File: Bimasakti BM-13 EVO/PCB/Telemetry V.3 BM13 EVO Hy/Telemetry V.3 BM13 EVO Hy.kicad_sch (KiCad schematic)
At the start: 7 parts, among them U1 ESP32-DEVKIT-V1, U2 74LVC125APW_118

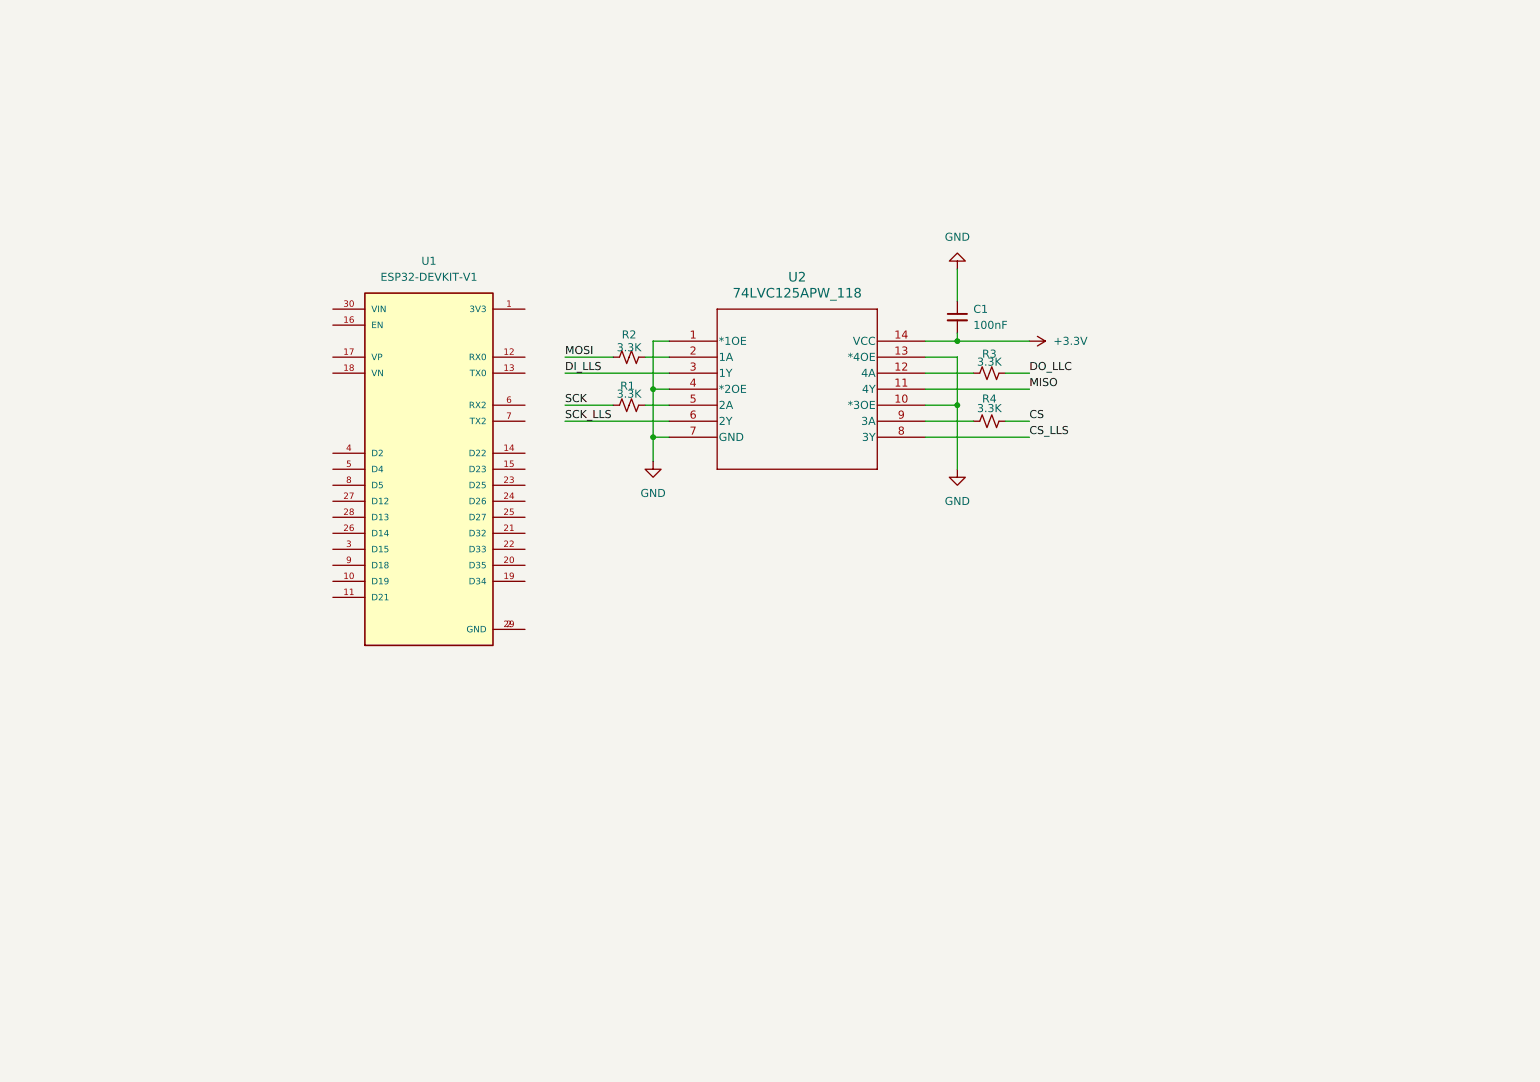
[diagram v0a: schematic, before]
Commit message: Arjun Ganti
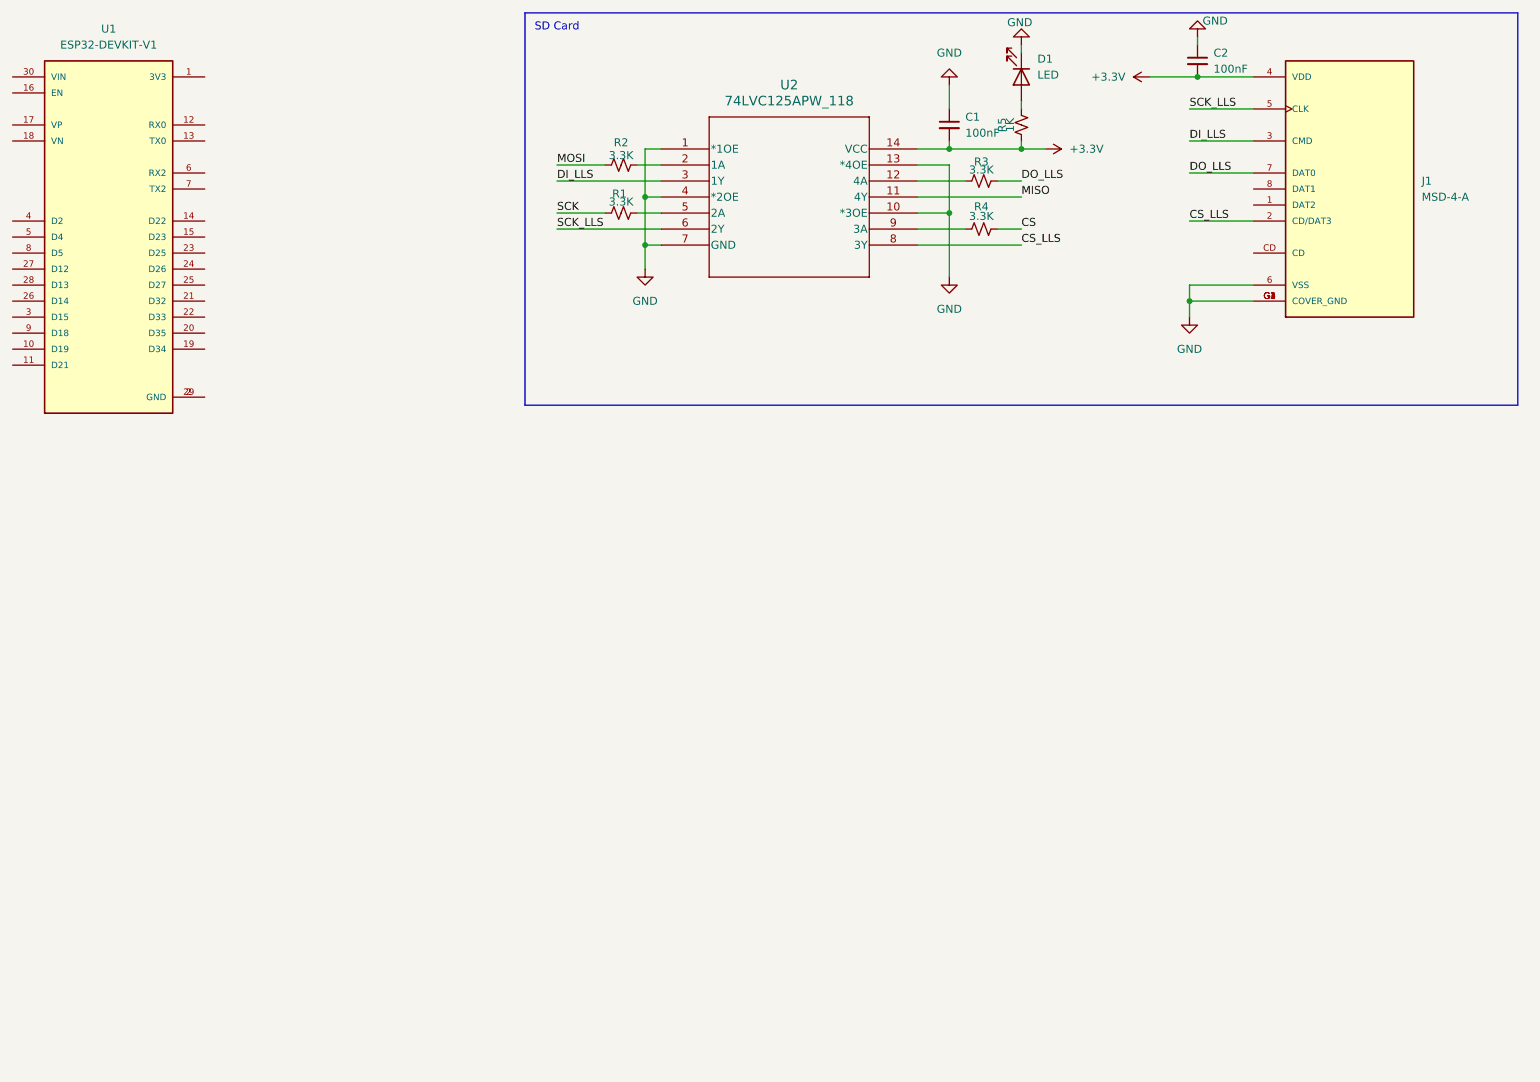
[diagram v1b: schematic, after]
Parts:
- added C2: 100nF, symbol Device:C_Small
- added D1: LED, symbol Device:LED
- added J1: MSD-4-A, MSD-4-A:CUI_MSD-4-A, symbol Micro SD Card Socket:MSD-4-A
- added R5: 1K, symbol Device:R_Small_US
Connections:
- net +3.3V: now also C2.2, J1.4 (VDD), R5.1
- net CS_LLS: now also J1.2 (CD/DAT3)
- net DI_LLS: now also J1.3 (CMD)
- net GND: now also C2.1, D1.1 (K), J1.6 (VSS), J1.G1 (COVER_GND), J1.G2 (COVER_GND), J1.G3 (COVER_GND), J1.G4 (COVER_GND)
- net SCK_LLS: now also J1.5 (CLK)
- net DO_LLC renamed DO_LLS
- net DO_LLS: now also J1.7 (DAT0)
- new net: D1.2 (A), R5.2
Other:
- note added: "SD Card"
- moved on the sheet: C1, R1, R2, R3, R4, U1, U2

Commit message: Arjun Telemetry hari 2
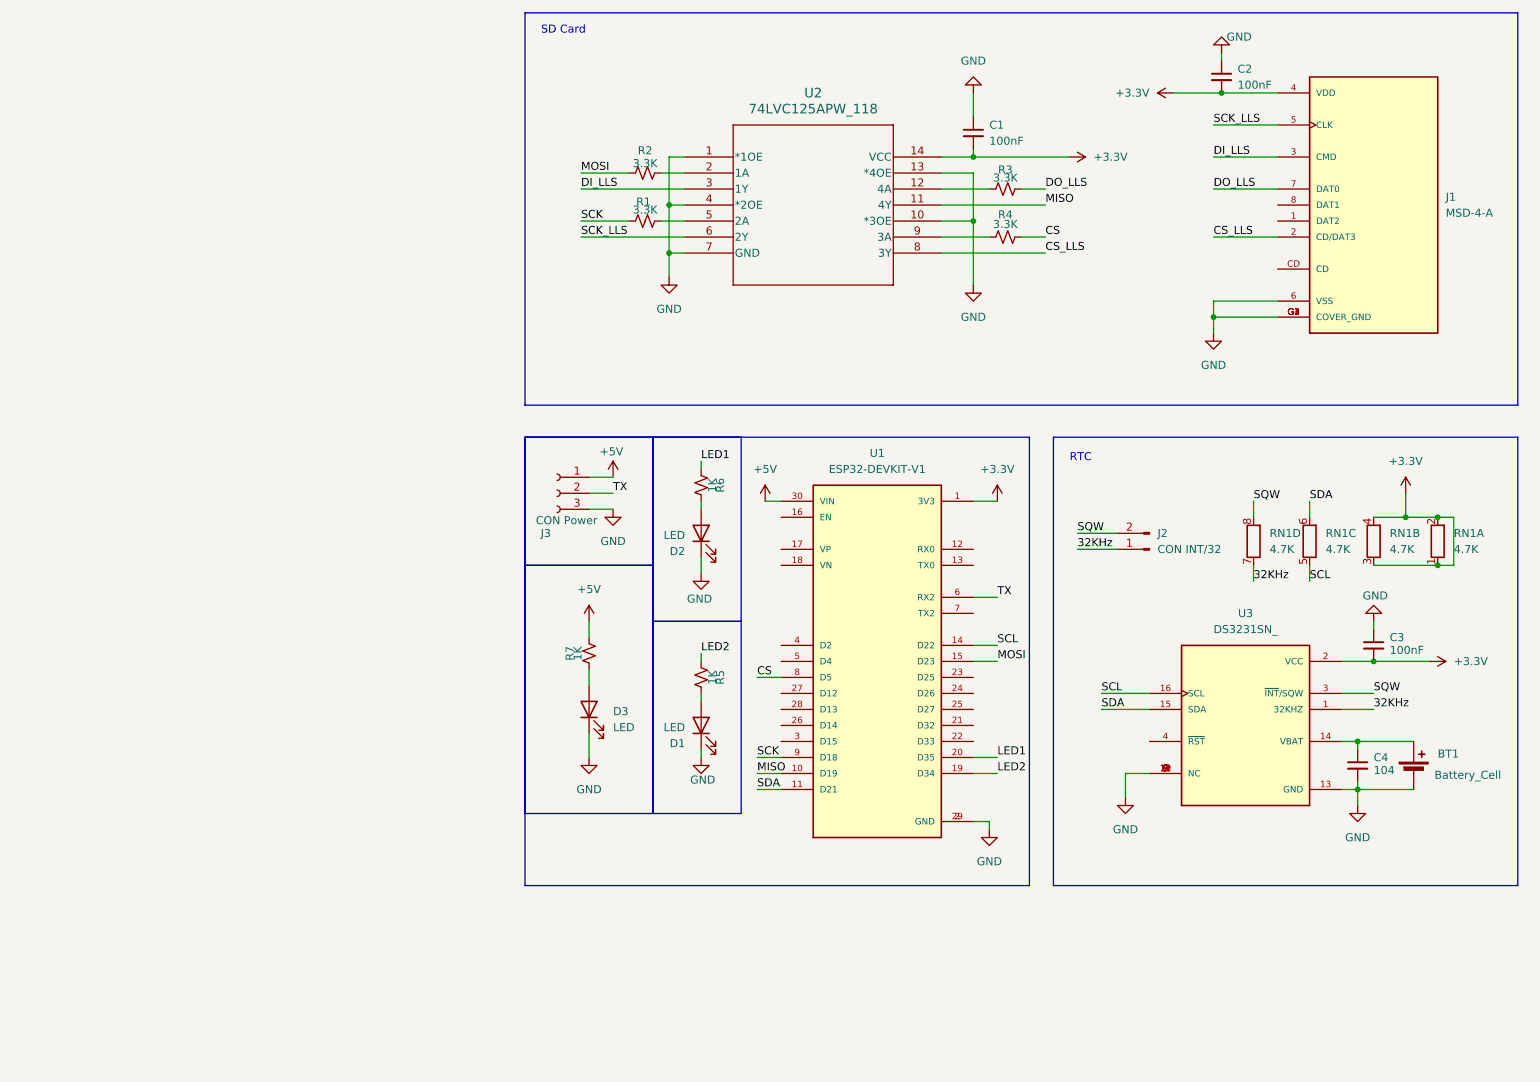
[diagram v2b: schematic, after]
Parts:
- added BT1: Battery_Cell, Battery:BatteryHolder_ComfortableElectronic_CH273-2450_1x2450, symbol Device:Battery_Cell
- added C3: 100nF, Capacitor_SMD:C_0603_1608Metric_Pad1.08x0.95mm_HandSolder, symbol Device:C_Small
- added C4: 104, Capacitor_SMD:C_0603_1608Metric_Pad1.08x0.95mm_HandSolder, symbol Device:C_Small
- added D2, D3: LED, LED_SMD:LED_0603_1608Metric_Pad1.05x0.95mm_HandSolder, symbol Device:LED
- added J2: CON INT/32, Connector_PinHeader_2.54mm:PinHeader_1x02_P2.54mm_Vertical, symbol Connector:Conn_01x02_Pin
- added J3: CON Power, Connector_JST:JST_XH_B3B-XH-A_1x03_P2.50mm_Vertical, symbol Connector:Conn_01x03_Socket
- added R6, R7: 1K, Resistor_SMD:R_0603_1608Metric_Pad0.98x0.95mm_HandSolder, symbol Device:R_Small_US
- added RN1: 4.7K, Resistor_SMD:R_Array_Convex_4x0603, symbol Device:R_Pack04_SIP_Split
- added U3: DS3231SN_, DS3231SN#:SOIC127P1032X265-16N, symbol DS3231SN_:DS3231SN_
- C1, C2: footprint (none) -> Capacitor_SMD:C_0603_1608Metric_Pad1.08x0.95mm_HandSolder
- D1: footprint (none) -> LED_SMD:LED_0603_1608Metric_Pad1.05x0.95mm_HandSolder
- J1: footprint MSD-4-A:CUI_MSD-4-A -> SDCard Socket:CUI_MSD-4-A
- R1, R2, R3, R4, R5: footprint (none) -> Resistor_SMD:R_0603_1608Metric_Pad0.98x0.95mm_HandSolder
- U1: footprint ESP32-DEVKIT-V1:MODULE_ESP32_DEVKIT_V1 -> ESP32:MODULE_ESP32_DEVKIT_V1
- U2: footprint TSSOP14_SOT402-1_NEX -> 74LVC125APW,118:TSSOP14_SOT402-1_NEX
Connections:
- net +3.3V: now also U1.1 (3V3), C3.2, RN1.1 (R1.1), RN1.2 (R1.2), RN1.3 (R2.1), RN1.4 (R2.2), U3.2 (VCC); no longer R5.1
- net CS: now also U1.8 (D5)
- net GND: now also U1.2 (GND), U1.29 (GND), BT1.2 (-), C3.1, C4.2, D2.1 (K), D3.1 (K), J3.3 (Pin_3), U3.10 (NC), U3.11 (NC), U3.12 (NC), U3.13 (GND), U3.5 (NC), U3.6 (NC), U3.7 (NC), U3.8 (NC), U3.9 (NC)
- net MISO: now also U1.10 (D19)
- net MOSI: now also U1.15 (D23)
- net SCK: now also U1.9 (D18)
- net SDA: now reaches U1.11 (D21)
- net SDA: now also RN1.6 (R3.2), U3.15 (SDA)
- net SCL: now reaches U1.14 (D22)
- net SCL: now also RN1.5 (R3.1), U3.16 (SCL)
- net LED2: now reaches U1.19 (D34)
- net LED2: now also R5.1
- net LED1: now reaches U1.20 (D35)
- net LED1: now also R6.1
- net +5V: now reaches U1.30 (VIN)
- net +5V: now also J3.1 (Pin_1), R7.2
- net TX: now reaches U1.6 (RX2)
- net TX: now also J3.2 (Pin_2)
- new net: BT1.1 (+), C4.1, U3.14 (VBAT)
- new net: D2.2 (A), R6.2
- new net: D3.2 (A), R7.1
- new net 32KHz: J2.1 (Pin_1), RN1.7 (R4.1), U3.1 (32KHZ)
- new net SQW: J2.2 (Pin_2), RN1.8 (R4.2), U3.3 (~{INT}/SQW)
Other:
- note added: "RTC"
- moved on the sheet: C1, C2, D1, J1, R1, R2, R3, R4, R5, U1, U2

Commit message: Telemetry
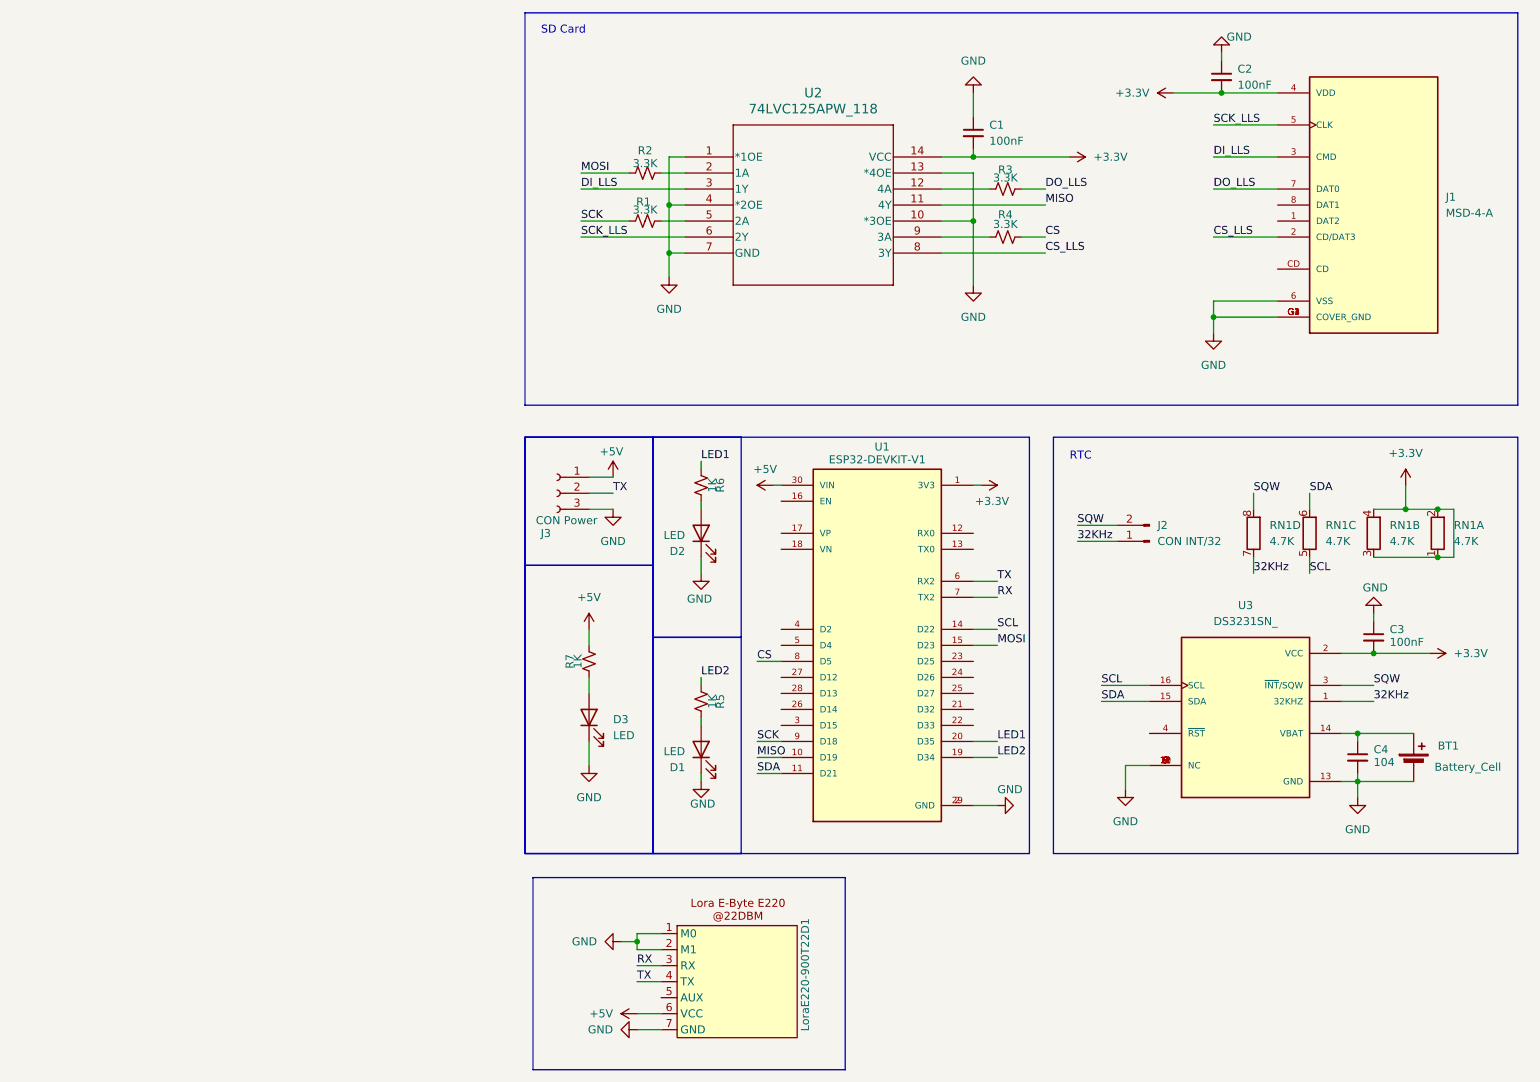
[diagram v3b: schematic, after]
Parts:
- added LoraE220-900T22D1: ~, Lora E220-900T22D:Lora E220-900T22D, symbol Lora:Lora_E220
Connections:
- net +5V: now also LoraE220-900T22D1.6 (VCC)
- net GND: now also LoraE220-900T22D1.1 (M0), LoraE220-900T22D1.2 (M1), LoraE220-900T22D1.7 (GND)
- net TX: now also LoraE220-900T22D1.4 (TX)
- net RX: now reaches U1.7 (TX2)
- net RX: now also LoraE220-900T22D1.3 (RX)
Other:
- moved on the sheet: BT1, C3, C4, D1, D3, J2, R5, R7, RN1A, RN1B, RN1C, RN1D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
